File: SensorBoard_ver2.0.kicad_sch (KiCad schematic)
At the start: 4 parts

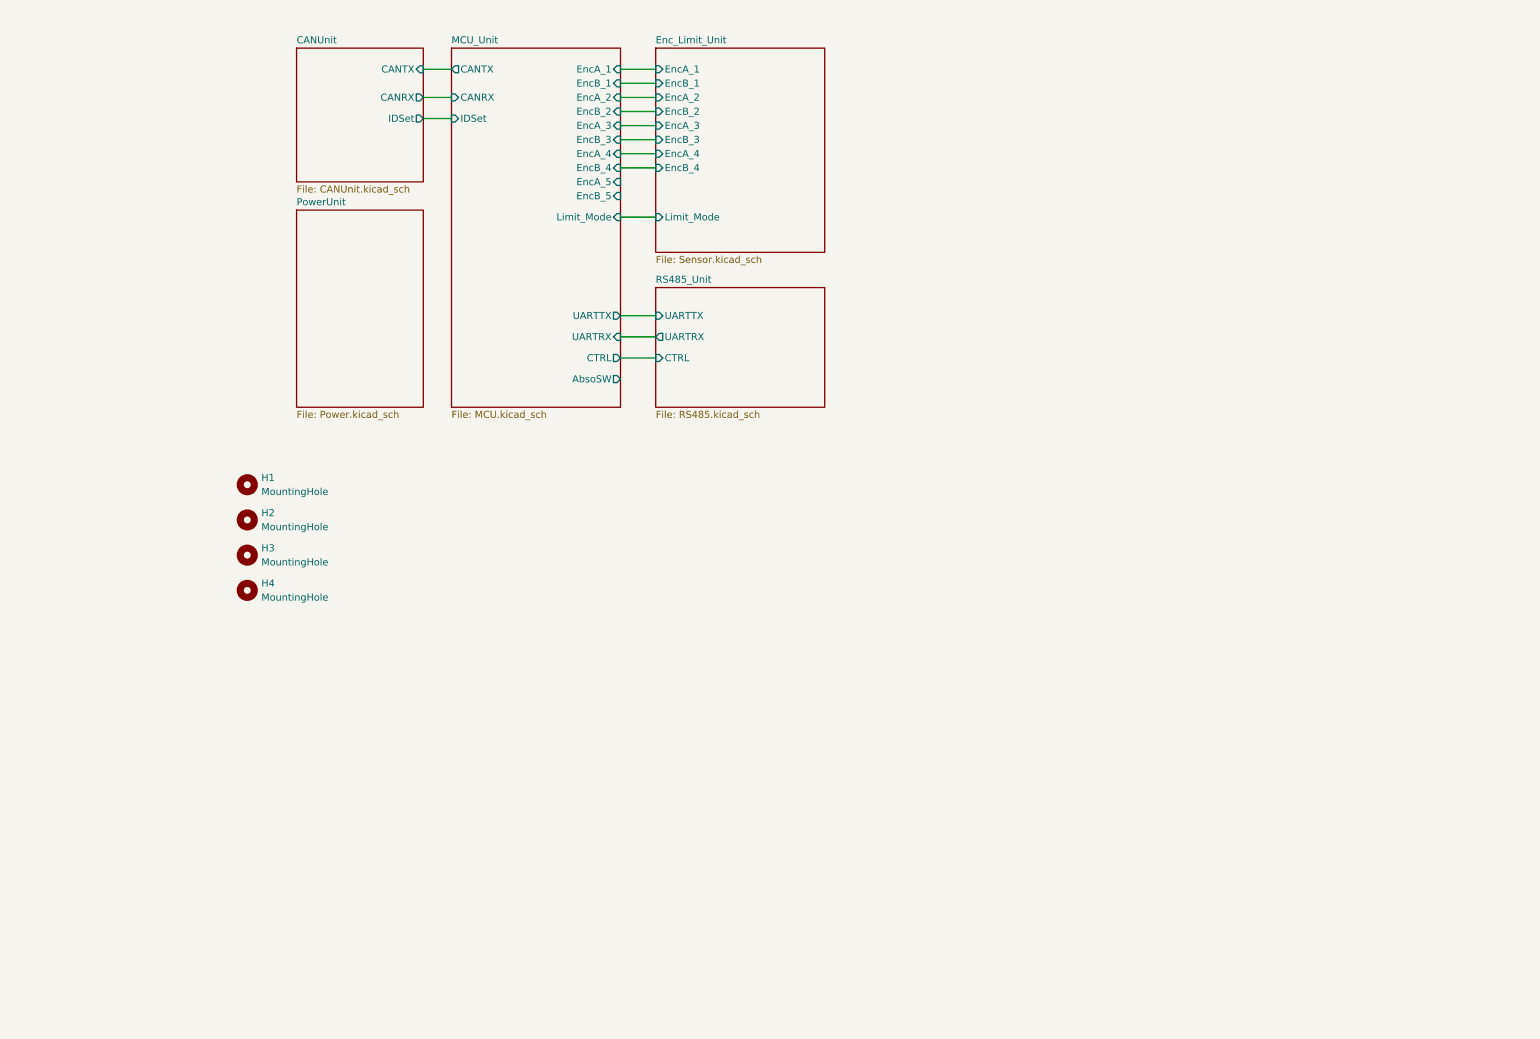
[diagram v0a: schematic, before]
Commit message: 回路図作った
リミットとエンコ共存いやかも
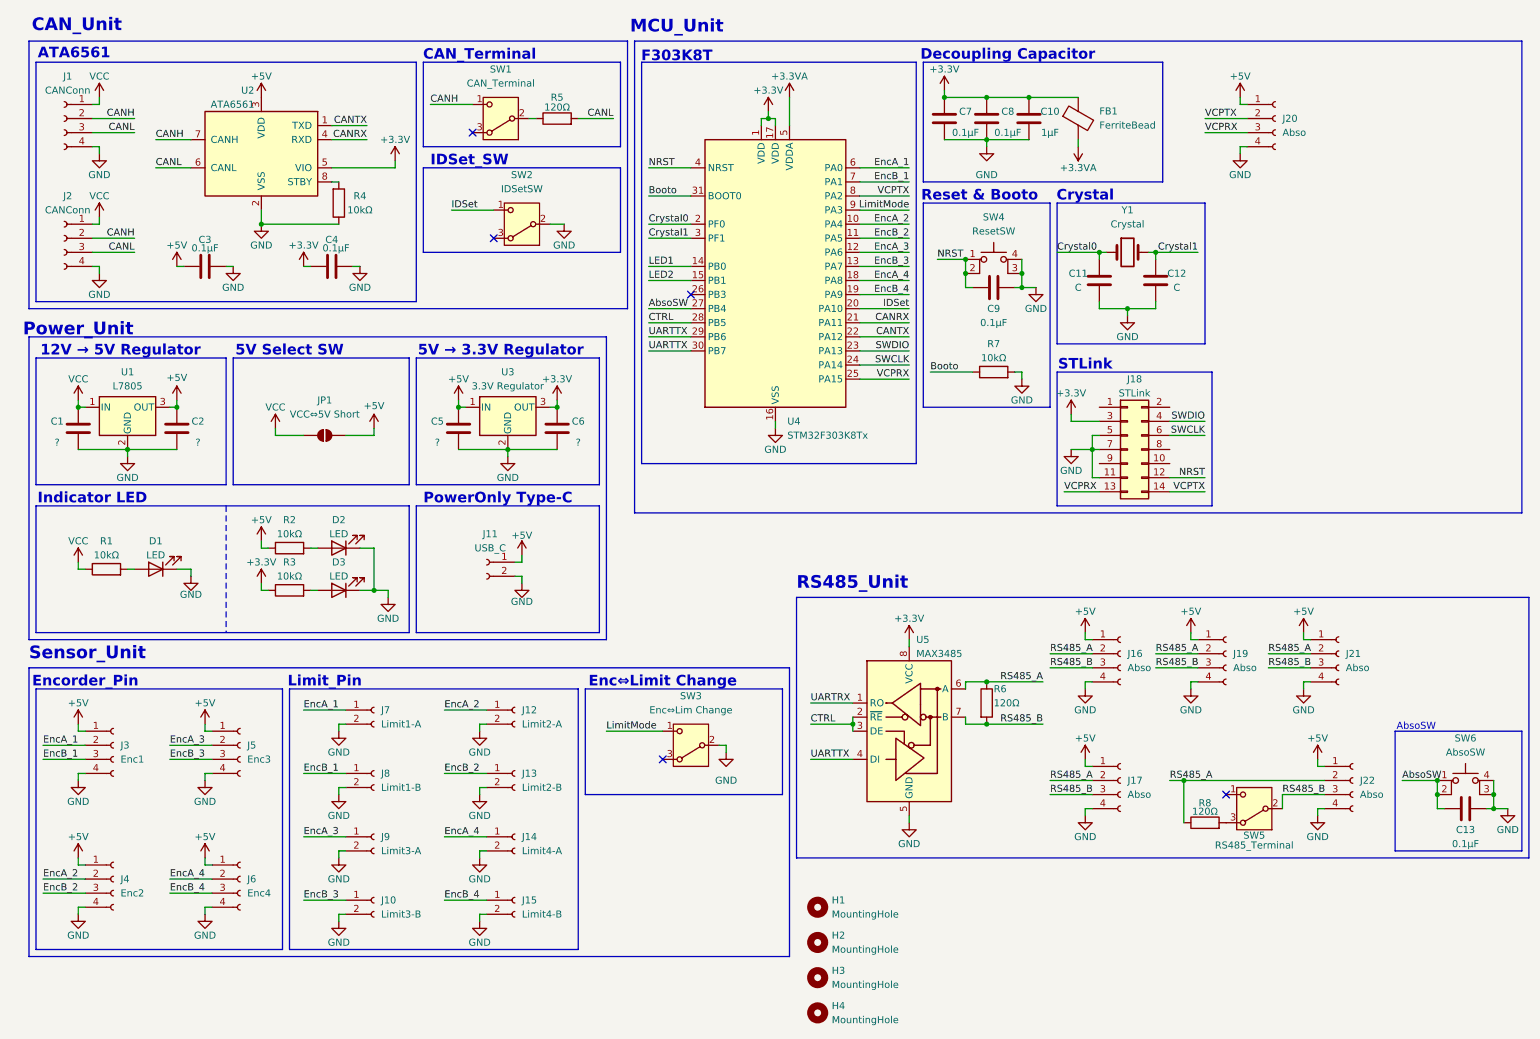
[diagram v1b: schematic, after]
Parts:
- added C1, C2, C5, C6: ?, Capacitor_SMD:C_0603_1608Metric, symbol Device:C
- added C10: 1μF, Capacitor_SMD:C_0603_1608Metric, symbol Device:C
- added C11, C12: C, Capacitor_SMD:C_0603_1608Metric, symbol Device:C
- added C13, C3, C4, C7, C8, C9: 0.1μF, Capacitor_SMD:C_0603_1608Metric, symbol Device:C
- added D1, D2, D3: LED, LED_SMD:LED_0603_1608Metric, symbol Device:LED
- added FB1: FerriteBead, Inductor_SMD:L_0603_1608Metric, symbol Device:FerriteBead
- added J1, J2: CANConn, Connector_JST:JST_XA_S04B-XASK-1_1x04_P2.50mm_Horizontal, symbol Connector:Conn_01x04_Socket
- added J10: Limit3-B, Connector_JST:JST_XA_B02B-XASK-1_1x02_P2.50mm_Vertical, symbol Connector:Conn_01x02_Socket
- added J11: USB_C, MyUSB_C:PowerOnlyUSB_C, symbol Connector:Conn_01x02_Socket
- added J12: Limit2-A, Connector_JST:JST_XA_B02B-XASK-1_1x02_P2.50mm_Vertical, symbol Connector:Conn_01x02_Socket
- added J13: Limit2-B, Connector_JST:JST_XA_B02B-XASK-1_1x02_P2.50mm_Vertical, symbol Connector:Conn_01x02_Socket
- added J14: Limit4-A, Connector_JST:JST_XA_B02B-XASK-1_1x02_P2.50mm_Vertical, symbol Connector:Conn_01x02_Socket
- added J15: Limit4-B, Connector_JST:JST_XA_B02B-XASK-1_1x02_P2.50mm_Vertical, symbol Connector:Conn_01x02_Socket
- added J16, J17, J19, J20, J21, J22: Abso, Connector_JST:JST_XA_S04B-XASK-1_1x04_P2.50mm_Horizontal, symbol Connector:Conn_01x04_Socket
- added J18: STLink, Connector_PinHeader_1.27mm:PinHeader_2x07_P1.27mm_Vertical_SMD, symbol Connector_Generic:Conn_02x07_Odd_Even
- added J3: Enc1, Connector_JST:JST_XA_S04B-XASK-1_1x04_P2.50mm_Horizontal, symbol Connector:Conn_01x04_Socket
- added J4: Enc2, Connector_JST:JST_XA_S04B-XASK-1_1x04_P2.50mm_Horizontal, symbol Connector:Conn_01x04_Socket
- added J5: Enc3, Connector_JST:JST_XA_S04B-XASK-1_1x04_P2.50mm_Horizontal, symbol Connector:Conn_01x04_Socket
- added J6: Enc4, Connector_JST:JST_XA_S04B-XASK-1_1x04_P2.50mm_Horizontal, symbol Connector:Conn_01x04_Socket
- added J7: Limit1-A, Connector_JST:JST_XA_B02B-XASK-1_1x02_P2.50mm_Vertical, symbol Connector:Conn_01x02_Socket
- added J8: Limit1-B, Connector_JST:JST_XA_B02B-XASK-1_1x02_P2.50mm_Vertical, symbol Connector:Conn_01x02_Socket
- added J9: Limit3-A, Connector_JST:JST_XA_B02B-XASK-1_1x02_P2.50mm_Vertical, symbol Connector:Conn_01x02_Socket
- added JP1: VCC⇔5V Short, Jumper:SolderJumper-2_P1.3mm_Open_RoundedPad1.0x1.5mm, symbol Jumper:SolderJumper_2_Open
- added R1, R2, R3, R4, R7: 10kΩ, Resistor_SMD:R_0603_1608Metric, symbol Device:R
- added R5: 120Ω, symbol Device:R
- added R6, R8: 120Ω, Resistor_SMD:R_0603_1608Metric, symbol Device:R
- added SW1: CAN_Terminal, Connector_PinHeader_2.54mm:PinHeader_1x03_P2.54mm_Vertical, symbol Switch:SW_Nidec_CAS-120A1
- added SW2: IDSetSW, Connector_PinHeader_2.54mm:PinHeader_1x03_P2.54mm_Vertical, symbol Switch:SW_Nidec_CAS-120A1
- added SW3: Enc⇔Lim Change, Connector_PinHeader_2.54mm:PinHeader_1x03_P2.54mm_Vertical, symbol Switch:SW_Nidec_CAS-120A1
- added SW4: ResetSW, symbol Switch:SW_MEC_5E
- added SW5: RS485_Terminal, Connector_PinHeader_2.54mm:PinHeader_1x03_P2.54mm_Vertical, symbol Switch:SW_Nidec_CAS-120A1
- added SW6: AbsoSW, symbol Switch:SW_MEC_5E
- added U1: L7805, Package_TO_SOT_SMD:TO-252-2, symbol Regulator_Linear:L7805
- added U2: ATA6561, Package_SO:SOIC-8_3.9x4.9mm_P1.27mm, symbol Interface_CAN_LIN:MCP2551-I-SN
- added U3: 3.3V Regulator, Package_TO_SOT_SMD:SOT-223, symbol Regulator_Linear:L7805
- added U4: STM32F303K8Tx, Package_QFP:LQFP-32_7x7mm_P0.8mm, symbol MCU_ST_STM32F3:STM32F303K8Tx
- added U5: MAX3485, Package_SO:SOIC-8_3.9x4.9mm_P1.27mm, symbol Interface_UART:MAX3485
- added Y1: Crystal, Crystal:Crystal_SMD_HC49-SD, symbol Device:Crystal
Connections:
- new net: R8.2, SW5.3 (A)
- new net: D3.2 (A), R3.2
- new net: D2.2 (A), R2.2
- new net: R5.1, SW1.2 (B)
- new net: D1.2 (A), R1.2
- new net: R4.2, U2.8 (STBY)
- new net +3.3V: C10.1, C4.1, C6.1, C7.1, C8.1, FB1.1, J18.3 (Pin_3), R3.1, U2.5 (VIO), U3.3 (OUT), U4.1 (VDD), U4.17 (VDD), U5.8 (VCC)
- new net +3.3VA: FB1.2, U4.5 (VDDA)
- new net +5V: C2.1, C3.1, C5.1, J11.1 (Pin_1), J16.1 (Pin_1), J17.1 (Pin_1), J19.1 (Pin_1), J20.1 (Pin_1), J21.1 (Pin_1), J22.1 (Pin_1), J3.1 (Pin_1), J4.1 (Pin_1), J5.1 (Pin_1), J6.1 (Pin_1), JP1.2 (B), R2.1, U1.3 (OUT), U2.3 (VDD), U3.1 (IN)
- new net AbsoSW: C13.2, SW6.1, SW6.2, U4.27 (PB4)
- new net Booto: R7.1, U4.31 (BOOT0)
- new net CANH: J1.2 (Pin_2), J2.2 (Pin_2), SW1.1 (C), U2.7 (CANH)
- new net CANL: J1.3 (Pin_3), J2.3 (Pin_3), R5.2, U2.6 (CANL)
- new net CANRX: U2.4 (RXD), U4.21 (PA11)
- new net CANTX: U2.1 (TXD), U4.22 (PA12)
- new net CTRL: U4.28 (PB5), U5.2 (~{RE}), U5.3 (DE)
- new net Crystal0: C11.1, U4.2 (PF0), Y1.1
- new net Crystal1: C12.1, U4.3 (PF1), Y1.2
- new net EncA_1: J3.2 (Pin_2), J7.1 (Pin_1), U4.6 (PA0)
- new net EncA_2: J12.1 (Pin_1), J4.2 (Pin_2), U4.10 (PA4)
- new net EncA_3: J5.2 (Pin_2), J9.1 (Pin_1), U4.12 (PA6)
- new net EncA_4: J14.1 (Pin_1), J6.2 (Pin_2), U4.18 (PA8)
- new net EncB_1: J3.3 (Pin_3), J8.1 (Pin_1), U4.7 (PA1)
- new net EncB_2: J13.1 (Pin_1), J4.3 (Pin_3), U4.11 (PA5)
- new net EncB_3: J10.1 (Pin_1), J5.3 (Pin_3), U4.13 (PA7)
- new net EncB_4: J15.1 (Pin_1), J6.3 (Pin_3), U4.19 (PA9)
- new net GND: C1.2, C10.2, C11.2, C12.2, C13.1, C2.2, C3.2, C4.2, C5.2, C6.2, C7.2, C8.2, C9.1, D1.1 (K), D2.1 (K), D3.1 (K), J1.4 (Pin_4), J10.2 (Pin_2), J11.2 (Pin_2), J12.2 (Pin_2), J13.2 (Pin_2), J14.2 (Pin_2), J15.2 (Pin_2), J16.4 (Pin_4), J17.4 (Pin_4), J18.11 (Pin_11), J18.5 (Pin_5), J18.7 (Pin_7), J19.4 (Pin_4), J2.4 (Pin_4), J20.4 (Pin_4), J21.4 (Pin_4), J22.4 (Pin_4), J3.4 (Pin_4), J4.4 (Pin_4), J5.4 (Pin_4), J6.4 (Pin_4), J7.2 (Pin_2), J8.2 (Pin_2), J9.2 (Pin_2), R4.1, R7.2, SW2.2 (B), SW3.2 (B), SW4.3 (K), SW4.4 (A), SW6.3 (K), SW6.4 (A), U1.2 (GND), U2.2 (VSS), U3.2 (GND), U4.16 (VSS), U4.32 (VSS), U5.5 (GND)
- new net IDSet: SW2.1 (C), U4.20 (PA10)
- new net LED1: U4.14 (PB0)
- new net LED2: U4.15 (PB1)
- new net LimitMode: SW3.1 (C), U4.9 (PA3)
- new net NRST: C9.2, J18.12 (Pin_12), SW4.1, SW4.2, U4.4 (NRST)
- new net RS485_A: J16.2 (Pin_2), J17.2 (Pin_2), J19.2 (Pin_2), J21.2 (Pin_2), J22.2 (Pin_2), R6.1, R8.1, U5.6 (A)
- new net RS485_B: J16.3 (Pin_3), J17.3 (Pin_3), J19.3 (Pin_3), J21.3 (Pin_3), J22.3 (Pin_3), R6.2, SW5.2 (B), U5.7 (B)
- new net SWCLK: J18.6 (Pin_6), U4.24 (PA14)
- new net SWDIO: J18.4 (Pin_4), U4.23 (PA13)
- new net UARTRX: U5.1 (RO)
- new net UARTTX: U4.29 (PB6), U4.30 (PB7), U5.4 (DI)
- new net VCC: C1.1, J1.1 (Pin_1), J2.1 (Pin_1), JP1.1 (A), R1.1, U1.1 (IN)
- new net VCPRX: J18.13 (Pin_13), J20.3 (Pin_3), U4.25 (PA15)
- new net VCPTX: J18.14 (Pin_14), J20.2 (Pin_2), U4.8 (PA2)
- no-connect marks 0 -> 5
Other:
- removed sheet CANUnit
- removed sheet Enc_Limit_Unit
- removed sheet MCU_Unit
- removed sheet PowerUnit
- removed sheet RS485_Unit
- note added: "12V → 5V Regulator"
- note added: "5V Select SW"
- note added: "5V → 3.3V Regulator"
- note added: "ATA6561"
- note added: "AbsoSW"
- note added: "CAN_Terminal"
- note added: "CAN_Unit"
- note added: "Crystal"
- note added: "Decoupling Capacitor"
- note added: "Encorder_Pin"
- note added: "Enc⇔Limit Change"
- note added: "F303K8T"
- note added: "IDSet_SW"
- note added: "Indicator LED"
- note added: "Limit_Pin"
- note added: "MCU_Unit"
- note added: "PowerOnly Type-C"
- note added: "Power_Unit"
- note added: "RS485_Unit"
- note added: "Reset & Booto"
- note added: "STLink"
- note added: "Sensor_Unit"
- title: (none) -> SensorBoard(Potato)_ver2.0
- moved on the sheet: H1, H2, H3, H4
